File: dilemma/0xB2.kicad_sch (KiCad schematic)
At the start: 105 parts, among them J1 USB_C_Receptacle_USB2.0, J101 trackball, J102 Serial, J103 Serial, J104 BATTERY_CONN_DEANS, J105 S3B-PH-SM4-TB(LF)(SN), J106 S3B-PH-SM4-TB(LF)(SN), J113 Cirque, J5 Conn_01x02, SW1 SW_Push, SW101 SW_Push, SW102 SW_Push, SW103 SW_Push, SW104 SW_Push, SW105 SW_Push, SW106 SW_Push, SW107 SW_Push, SW108 SW_Push, SW109 SW_Push, SW110 SW_SPST, SW111 SW_SPST, SW112 SW_Push, SW113 SW_Push, SW114 SW_Push, SW115 SW_Push, SW116 SW_Push, SW117 SW_Push, SW118 SW_Push, SW119 SW_Push, SW2 SW_Push, U1 RP2040, U2 GD25Q80CEIGR, U3 XC6210B332MR-G, Y1 Crystal_GND24

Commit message: jlc parts
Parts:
- D101, D102, D103, D104, D105, D106, D107, D108, D109, D110, D111, D112, D113, D114, D115, D116, D117: footprint local-libraries:D_0402_1005Metric_bkb -> local-libraries:D_1206_handsolder_reversible
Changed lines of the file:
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@@
       (effects (font (size 1.27 1.27)) (justify right))
     )
-    (property "Footprint" "local-libraries:D_0402_1005Metric_bkb" (id 2) (at 388.62 48.26 0)
+    (property "Footprint" "local-libraries:D_1206_handsolder_reversible" (id 2) (at 388.62 48.26 0)
       (effects (font (size 1.27 1.27)) hide)
     )
@@
       (effects (font (size 1.27 1.27)) (justify right))
     )
-    (property "Footprint" "local-libraries:D_0402_1005Metric_bkb" (id 2) (at 415.29 58.42 0)
+    (property "Footprint" "local-libraries:D_1206_handsolder_reversible" (id 2) (at 415.29 58.42 0)
       (effects (font (size 1.27 1.27)) hide)
     )
@@
     (property "Reference" "D116" (id 0) (at 534.67 46.99 0))
     (property "Value" "D" (id 1) (at 534.67 49.53 0))
-    (property "Footprint" "local-libraries:D_0402_1005Metric_bkb" (id 2) (at 534.67 53.34 0)
+    (property "Footprint" "local-libraries:D_1206_handsolder_reversible" (id 2) (at 534.67 53.34 0)
       (effects (font (size 1.27 1.27)) hide)
     )
@@
       (effects (font (size 1.27 1.27)) (justify right))
     )
-    (property "Footprint" "local-libraries:D_0402_1005Metric_bkb" (id 2) (at 468.63 48.26 0)
+    (property "Footprint" "local-libraries:D_1206_handsolder_reversible" (id 2) (at 468.63 48.26 0)
       (effects (font (size 1.27 1.27)) hide)
     )
@@
     (property "Reference" "D117" (id 0) (at 548.64 46.99 0))
     (property "Value" "D" (id 1) (at 548.64 49.53 0))
-    (property "Footprint" "local-libraries:D_0402_1005Metric_bkb" (id 2) (at 548.64 53.34 0)
+    (property "Footprint" "local-libraries:D_1206_handsolder_reversible" (id 2) (at 548.64 53.34 0)
       (effects (font (size 1.27 1.27)) hide)
     )
@@
       (effects (font (size 1.27 1.27)) (justify right))
     )
-    (property "Footprint" "local-libraries:D_0402_1005Metric_bkb" (id 2) (at 441.96 38.1 0)
+    (property "Footprint" "local-libraries:D_1206_handsolder_reversible" (id 2) (at 441.96 38.1 0)
       (effects (font (size 1.27 1.27)) hide)
     )
@@
       (effects (font (size 1.27 1.27)) (justify right))
     )
-    (property "Footprint" "local-libraries:D_0402_1005Metric_bkb" (id 2) (at 415.29 48.26 0)
+    (property "Footprint" "local-libraries:D_1206_handsolder_reversible" (id 2) (at 415.29 48.26 0)
       (effects (font (size 1.27 1.27)) hide)
     )
@@
       (effects (font (size 1.27 1.27)) (justify right))
     )
-    (property "Footprint" "local-libraries:D_0402_1005Metric_bkb" (id 2) (at 415.29 38.1 0)
+    (property "Footprint" "local-libraries:D_1206_handsolder_reversible" (id 2) (at 415.29 38.1 0)
       (effects (font (size 1.27 1.27)) hide)
     )
@@
       (effects (font (size 1.27 1.27)) (justify right))
     )
-    (property "Footprint" "local-libraries:D_0402_1005Metric_bkb" (id 2) (at 468.63 38.1 0)
+    (property "Footprint" "local-libraries:D_1206_handsolder_reversible" (id 2) (at 468.63 38.1 0)
       (effects (font (size 1.27 1.27)) hide)
     )
@@
       (effects (font (size 1.27 1.27)) (justify right))
     )
-    (property "Footprint" "local-libraries:D_0402_1005Metric_bkb" (id 2) (at 388.62 38.1 0)
+    (property "Footprint" "local-libraries:D_1206_handsolder_reversible" (id 2) (at 388.62 38.1 0)
       (effects (font (size 1.27 1.27)) hide)
     )
@@
       (effects (font (size 1.27 1.27)) (justify right))
     )
-    (property "Footprint" "local-libraries:D_0402_1005Metric_bkb" (id 2) (at 495.3 48.26 0)
+    (property "Footprint" "local-libraries:D_1206_handsolder_reversible" (id 2) (at 495.3 48.26 0)
       (effects (font (size 1.27 1.27)) hide)
     )
@@
       (effects (font (size 1.27 1.27)) (justify right))
     )
-    (property "Footprint" "local-libraries:D_0402_1005Metric_bkb" (id 2) (at 468.63 58.42 0)
+    (property "Footprint" "local-libraries:D_1206_handsolder_reversible" (id 2) (at 468.63 58.42 0)
       (effects (font (size 1.27 1.27)) hide)
     )
@@
       (effects (font (size 1.27 1.27)) (justify right))
     )
-    (property "Footprint" "local-libraries:D_0402_1005Metric_bkb" (id 2) (at 441.96 58.42 0)
+    (property "Footprint" "local-libraries:D_1206_handsolder_reversible" (id 2) (at 441.96 58.42 0)
       (effects (font (size 1.27 1.27)) hide)
     )
@@
       (effects (font (size 1.27 1.27)) (justify right))
     )
-    (property "Footprint" "local-libraries:D_0402_1005Metric_bkb" (id 2) (at 388.62 58.42 0)
+    (property "Footprint" "local-libraries:D_1206_handsolder_reversible" (id 2) (at 388.62 58.42 0)
       (effects (font (size 1.27 1.27)) hide)
     )
@@
       (effects (font (size 1.27 1.27)) (justify right))
     )
-    (property "Footprint" "local-libraries:D_0402_1005Metric_bkb" (id 2) (at 441.96 48.26 0)
+    (property "Footprint" "local-libraries:D_1206_handsolder_reversible" (id 2) (at 441.96 48.26 0)
       (effects (font (size 1.27 1.27)) hide)
     )
@@
       (effects (font (size 1.27 1.27)) (justify right))
     )
-    (property "Footprint" "local-libraries:D_0402_1005Metric_bkb" (id 2) (at 495.3 38.1 0)
+    (property "Footprint" "local-libraries:D_1206_handsolder_reversible" (id 2) (at 495.3 38.1 0)
       (effects (font (size 1.27 1.27)) hide)
     )
@@
       (effects (font (size 1.27 1.27)) (justify right))
     )
-    (property "Footprint" "local-libraries:D_0402_1005Metric_bkb" (id 2) (at 495.3 58.42 0)
+    (property "Footprint" "local-libraries:D_1206_handsolder_reversible" (id 2) (at 495.3 58.42 0)
       (effects (font (size 1.27 1.27)) hide)
     )
@@
     )
     (path "/884b30ea-af8f-4f82-a557-df4823436067"
-      (reference "D101") (unit 1) (value "D") (footprint "local-libraries:D_0402_1005Metric_bkb")
+      (reference "D101") (unit 1) (value "D") (footprint "local-libraries:D_1206_handsolder_reversible")
     )
     (path "/1336502c-11bd-4ec2-9aca-20ce8fd7c351"
-      (reference "D102") (unit 1) (value "D") (footprint "local-libraries:D_0402_1005Metric_bkb")
+      (reference "D102") (unit 1) (value "D") (footprint "local-libraries:D_1206_handsolder_reversible")
     )
     (path "/d9c9a498-33d2-4069-be67-c993eabe1d55"
-      (reference "D103") (unit 1) (value "D") (footprint "local-libraries:D_0402_1005Metric_bkb")
+      (reference "D103") (unit 1) (value "D") (footprint "local-libraries:D_1206_handsolder_reversible")
     )
     (path "/7ad70d78-f911-4e78-bfa3-eb4384fdc5b5"
-      (reference "D104") (unit 1) (value "D") (footprint "local-libraries:D_0402_1005Metric_bkb")
+      (reference "D104") (unit 1) (value "D") (footprint "local-libraries:D_1206_handsolder_reversible")
     )
     (path "/748aaee6-99ae-41ad-8caa-46dcb39df129"
-      (reference "D105") (unit 1) (value "D") (footprint "local-libraries:D_0402_1005Metric_bkb")
+      (reference "D105") (unit 1) (value "D") (footprint "local-libraries:D_1206_handsolder_reversible")
     )
     (path "/1f9097e7-c345-4ea0-87cd-6931bd3e5e20"
-      (reference "D106") (unit 1) (value "D") (footprint "local-libraries:D_0402_1005Metric_bkb")
+      (reference "D106") (unit 1) (value "D") (footprint "local-libraries:D_1206_handsolder_reversible")
     )
     (path "/6a7769c3-c80d-4f67-890e-9d198d478ddd"
-      (reference "D107") (unit 1) (value "D") (footprint "local-libraries:D_0402_1005Metric_bkb")
+      (reference "D107") (unit 1) (value "D") (footprint "local-libraries:D_1206_handsolder_reversible")
     )
     (path "/dc672fc4-349f-4386-9438-aaaac984aa5b"
-      (reference "D108") (unit 1) (value "D") (footprint "local-libraries:D_0402_1005Metric_bkb")
+      (reference "D108") (unit 1) (value "D") (footprint "local-libraries:D_1206_handsolder_reversible")
     )
     (path "/d9191217-fb4c-4445-8d6b-28ba96ed5884"
-      (reference "D109") (unit 1) (value "D") (footprint "local-libraries:D_0402_1005Metric_bkb")
+      (reference "D109") (unit 1) (value "D") (footprint "local-libraries:D_1206_handsolder_reversible")
     )
     (path "/7d590ff0-32de-4f01-bf4c-caa51c97e2a2"
-      (reference "D110") (unit 1) (value "D") (footprint "local-libraries:D_0402_1005Metric_bkb")
+      (reference "D110") (unit 1) (value "D") (footprint "local-libraries:D_1206_handsolder_reversible")
     )
     (path "/2ecc83c5-7c71-4e10-83c8-795f7b03e775"
-      (reference "D111") (unit 1) (value "D") (footprint "local-libraries:D_0402_1005Metric_bkb")
+      (reference "D111") (unit 1) (value "D") (footprint "local-libraries:D_1206_handsolder_reversible")
     )
     (path "/b134eb71-28da-4fab-b4ff-66250b349fbc"
-      (reference "D112") (unit 1) (value "D") (footprint "local-libraries:D_0402_1005Metric_bkb")
+      (reference "D112") (unit 1) (value "D") (footprint "local-libraries:D_1206_handsolder_reversible")
     )
     (path "/dc6cb566-6bf9-4b64-8af9-7dc0b2417d25"
-      (reference "D113") (unit 1) (value "D") (footprint "local-libraries:D_0402_1005Metric_bkb")
+      (reference "D113") (unit 1) (value "D") (footprint "local-libraries:D_1206_handsolder_reversible")
     )
     (path "/a225e9fd-6545-4110-8e72-7e9c999e5896"
-      (reference "D114") (unit 1) (value "D") (footprint "local-libraries:D_0402_1005Metric_bkb")
+      (reference "D114") (unit 1) (value "D") (footprint "local-libraries:D_1206_handsolder_reversible")
     )
     (path "/fab6e5d8-40f2-4d6a-a034-ef09d49a2969"
-      (reference "D115") (unit 1) (value "D") (footprint "local-libraries:D_0402_1005Metric_bkb")
+      (reference "D115") (unit 1) (value "D") (footprint "local-libraries:D_1206_handsolder_reversible")
     )
     (path "/20d20a6c-03cf-4a4c-8a77-7b10171706e4"
-      (reference "D116") (unit 1) (value "D") (footprint "local-libraries:D_0402_1005Metric_bkb")
+      (reference "D116") (unit 1) (value "D") (footprint "local-libraries:D_1206_handsolder_reversible")
     )
     (path "/5341f75f-445e-45d6-8d7c-693459db4b8f"
-      (reference "D117") (unit 1) (value "D") (footprint "local-libraries:D_0402_1005Metric_bkb")
+      (reference "D117") (unit 1) (value "D") (footprint "local-libraries:D_1206_handsolder_reversible")
     )
     (path "/ce9365fe-085a-4731-86d8-fc3e6b16f716"

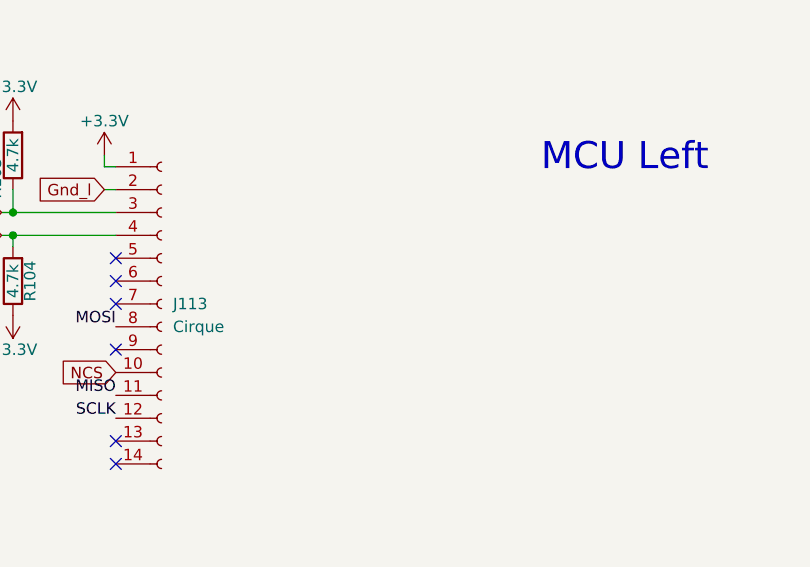
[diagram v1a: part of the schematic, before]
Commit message: spi breakout
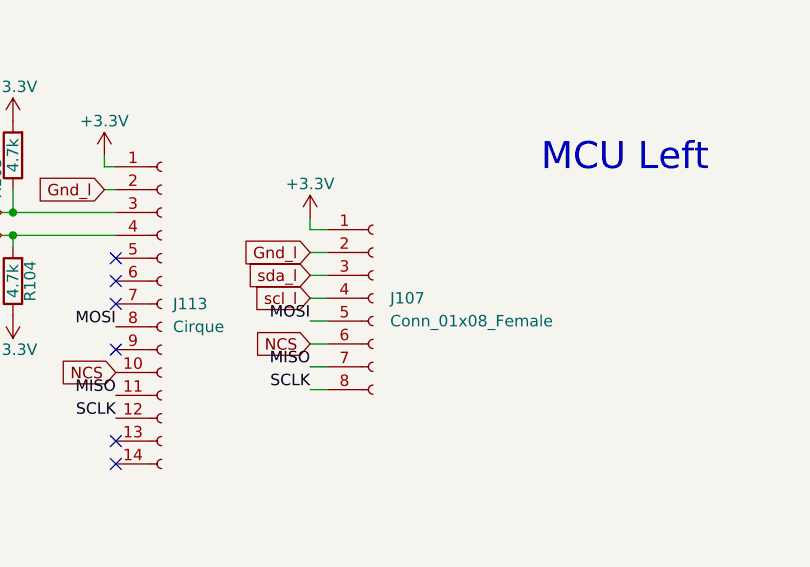
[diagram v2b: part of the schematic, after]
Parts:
- added J107: Conn_01x08_Female, local-libraries:1x08 smd reversible, symbol Connector:Conn_01x08_Female
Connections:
- net +3V3: now also J107.1 (Pin_1)
- net GND: now also J107.2 (Pin_2)
- net NCS: now also J107.6 (Pin_6)
- net miso_l: now also J107.7 (Pin_7)
- net mosi_l: now also J107.5 (Pin_5)
- net sc_l: now also J107.8 (Pin_8)
- net scl_l: now also J107.4 (Pin_4)
- net sda_l: now also J107.3 (Pin_3)
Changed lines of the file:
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@@
     (stroke (width 0) (type default) (color 0 0 0 0))
   )
+  (wire (pts (xy 339.725 90.805) (xy 337.82 90.805))
+    (stroke (width 0) (type default) (color 0 0 0 0))
+  )
   (wire (pts (xy 690.88 133.985) (xy 690.88 108.585))
     (stroke (width 0) (type default) (color 0 0 0 0))
@@
     (stroke (width 0) (type solid) (color 0 0 0 0))
   )
+  (wire (pts (xy 337.82 106.045) (xy 339.725 106.045))
+    (stroke (width 0) (type default) (color 0 0 0 0))
+  )
   (wire (pts (xy 101.6 175.26) (xy 101.6 176.53))
     (stroke (width 0) (type default) (color 0 0 0 0))
@@
     (stroke (width 0) (type default) (color 0 0 0 0))
   )
+  (wire (pts (xy 337.82 90.805) (xy 337.82 89.535))
+    (stroke (width 0) (type default) (color 0 0 0 0))
+  )
   (wire (pts (xy 46.355 160.655) (xy 55.245 160.655))
     (stroke (width 0) (type default) (color 0 0 0 0))
@@
     (stroke (width 0) (type default) (color 0 0 0 0))
   )
+  (wire (pts (xy 337.82 98.425) (xy 339.725 98.425))
+    (stroke (width 0) (type default) (color 0 0 0 0))
+  )
   (wire (pts (xy 445.77 48.26) (xy 449.58 48.26))
     (stroke (width 0) (type default) (color 0 0 0 0))
@@
     (stroke (width 0) (type default) (color 0 0 0 0))
   )
+  (wire (pts (xy 337.82 95.885) (xy 339.725 95.885))
+    (stroke (width 0) (type default) (color 0 0 0 0))
+  )
   (wire (pts (xy 415.925 150.495) (xy 415.925 147.32))
     (stroke (width 0) (type default) (color 0 0 0 0))
@@
     (stroke (width 0) (type default) (color 0 0 0 0))
   )
+  (wire (pts (xy 337.82 103.505) (xy 339.725 103.505))
+    (stroke (width 0) (type default) (color 0 0 0 0))
+  )
   (wire (pts (xy 304.8 88.9) (xy 316.23 88.9))
     (stroke (width 0) (type default) (color 0 0 0 0))
@@
     (stroke (width 0) (type default) (color 0 0 0 0))
   )
+  (wire (pts (xy 337.82 93.345) (xy 339.725 93.345))
+    (stroke (width 0) (type default) (color 0 0 0 0))
+  )
   (wire (pts (xy 661.035 133.985) (xy 661.035 131.445))
     (stroke (width 0) (type default) (color 0 0 0 0))
@@
     (stroke (width 0) (type default) (color 0 0 0 0))
   )
+  (wire (pts (xy 337.82 108.585) (xy 339.725 108.585))
+    (stroke (width 0) (type default) (color 0 0 0 0))
+  )
   (wire (pts (xy 101.6 184.15) (xy 101.6 185.42))
     (stroke (width 0) (type default) (color 0 0 0 0))
@@
     (stroke (width 0) (type default) (color 0 0 0 0))
   )
+  (wire (pts (xy 337.82 100.965) (xy 339.725 100.965))
+    (stroke (width 0) (type default) (color 0 0 0 0))
+  )
   (wire (pts (xy 182.88 71.12) (xy 191.77 71.12))
     (stroke (width 0) (type default) (color 0 0 0 0))
@@
     (effects (font (size 1.27 1.27)) (justify right bottom))
   )
+  (label "MOSI" (at 337.82 100.965 180)
+    (effects (font (size 1.27 1.27)) (justify right bottom))
+  )
   (label "QSPI_D2" (at 111.76 68.58 0)
     (effects (font (size 1.27 1.27)) (justify left bottom))
@@
     (effects (font (size 1.27 1.27)) (justify right bottom))
   )
+  (label "SCLK" (at 337.82 108.585 180)
+    (effects (font (size 1.27 1.27)) (justify right bottom))
+  )
   (label "QSPI_~{CS}" (at 218.44 129.54 0)
     (effects (font (size 1.27 1.27)) (justify left bottom))
@@
     (effects (font (size 1.27 1.27)) (justify right bottom))
   )
+  (label "MISO" (at 337.82 106.045 180)
+    (effects (font (size 1.27 1.27)) (justify right bottom))
+  )
   (label "QSPI_~{CS}" (at 46.355 160.655 0)
     (effects (font (size 1.27 1.27)) (justify left bottom))
@@
     )
   )
+  (global_label "sda_l" (shape input) (at 337.82 95.885 180)
+    (effects (font (size 1.27 1.27)) (justify right))
+    (property "Intersheet References" "${INTERSHEET_REFS}" (id 0) (at 308.61 41.275 0)
+      (effects (font (size 1.27 1.27)) hide)
+    )
+  )
   (global_label "Rst_l" (shape input) (at 445.77 102.235 180)
     (effects (font (size 1.27 1.27)) (justify right))
@@
     )
   )
+  (global_label "Gnd_l" (shape input) (at 337.82 93.345 180)
+    (effects (font (size 1.27 1.27)) (justify right))
+    (property "Intersheet References" "${INTERSHEET_REFS}" (id 0) (at 461.01 163.195 0)
+      (effects (font (size 1.27 1.27)) hide)
+    )
+  )
   (global_label "Gnd_l" (shape input) (at 228.6 46.99 180)
     (effects (font (size 1.27 1.27)) (justify right))
@@
     )
   )
+  (global_label "NCS" (shape input) (at 337.82 103.505 180)
+    (effects (font (size 1.27 1.27)) (justify right))
+    (property "Intersheet References" "${INTERSHEET_REFS}" (id 0) (at 333.3507 103.4256 0)
+      (effects (font (size 1.27 1.27)) (justify right) hide)
+    )
+  )
   (global_label "scl_l" (shape input) (at 228.6 52.07 180)
     (effects (font (size 1.27 1.27)) (justify right))
@@
     )
   )
+  (global_label "scl_l" (shape input) (at 337.82 98.425 180)
+    (effects (font (size 1.27 1.27)) (justify right))
+    (property "Intersheet References" "${INTERSHEET_REFS}" (id 0) (at 308.61 43.815 0)
+      (effects (font (size 1.27 1.27)) hide)
+    )
+  )
   (symbol (lib_id "Connector:Conn_01x02_Female") (at 551.815 123.825 0) (unit 1)
     (in_bom yes) (on_board yes)
@@
     (pin "T")
   )
+  (symbol (lib_id "power:+3.3V") (at 337.82 89.535 0) (unit 1)
+    (in_bom yes) (on_board yes)
+    (property "Reference" "#PWR0121" (id 0) (at 337.82 93.345 0)
+      (effects (font (size 1.27 1.27)) hide)
+    )
+    (property "Value" "+3.3V" (id 1) (at 337.82 85.725 0))
+    (property "Footprint" "" (id 2) (at 337.82 89.535 0)
+      (effects (font (size 1.27 1.27)) hide)
+    )
+    (property "Datasheet" "" (id 3) (at 337.82 89.535 0)
+      (effects (font (size 1.27 1.27)) hide)
+    )
+    (pin "1")
+  )
   (symbol (lib_id "Device:C") (at 121.92 180.34 0) (unit 1)
     (in_bom yes) (on_board yes)
@@
     (pin "2")
   )
+  (symbol (lib_id "Connector:Conn_01x08_Female") (at 344.805 98.425 0) (unit 1)
+    (in_bom yes) (on_board yes) (fields_autoplaced)
+    (property "Reference" "J107" (id 0) (at 346.71 98.4249 0)
+      (effects (font (size 1.27 1.27)) (justify left))
+    )
+    (property "Value" "Conn_01x08_Female" (id 1) (at 346.71 100.9649 0)
+      (effects (font (size 1.27 1.27)) (justify left))
+    )
+    (property "Footprint" "local-libraries:1x08 smd reversible" (id 2) (at 344.805 98.425 0)
+      (effects (font (size 1.27 1.27)) hide)
+    )
+    (property "Datasheet" "~" (id 3) (at 344.805 98.425 0)
+      (effects (font (size 1.27 1.27)) hide)
+    )
+    (pin "1")
+    (pin "2")
+    (pin "3")
+    (pin "4")
+    (pin "5")
+    (pin "6")
+    (pin "7")
+    (pin "8")
+  )
   (symbol (lib_id "Device:C") (at 111.76 101.6 0) (unit 1)
     (in_bom yes) (on_board yes)
@@
       (reference "#PWR0120") (unit 1) (value "+3.3V") (footprint "")
     )
+    (path "/351416fe-369a-4fca-8e5f-0d3c65de7c2e"
+      (reference "#PWR0121") (unit 1) (value "+3.3V") (footprint "")
+    )
     (path "/4a21e78b-0ab0-4b88-8132-9b174e045719"
       (reference "C1") (unit 1) (value "1µ") (footprint "Capacitor_SMD:C_0603_1608Metric")
@@
       (reference "J106") (unit 1) (value "S3B-PH-SM4-TB(LF)(SN)") (footprint "local-libraries:JST_SH_BM02B-SRSS-TB_1x02-1MP_P1.00mm_Vertical")
     )
+    (path "/8990af71-d145-4ceb-afc3-ba328829719a"
+      (reference "J107") (unit 1) (value "Conn_01x08_Female") (footprint "local-libraries:1x08 smd reversible")
+    )
     (path "/eeb6b826-bc65-4571-ab3b-1b47a831da34"
